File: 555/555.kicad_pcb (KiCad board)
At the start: 2 copper layers, 10 parts, among them J1 Conn_01x03_Pin, U1 LM555xM, U2 TSOP17xx

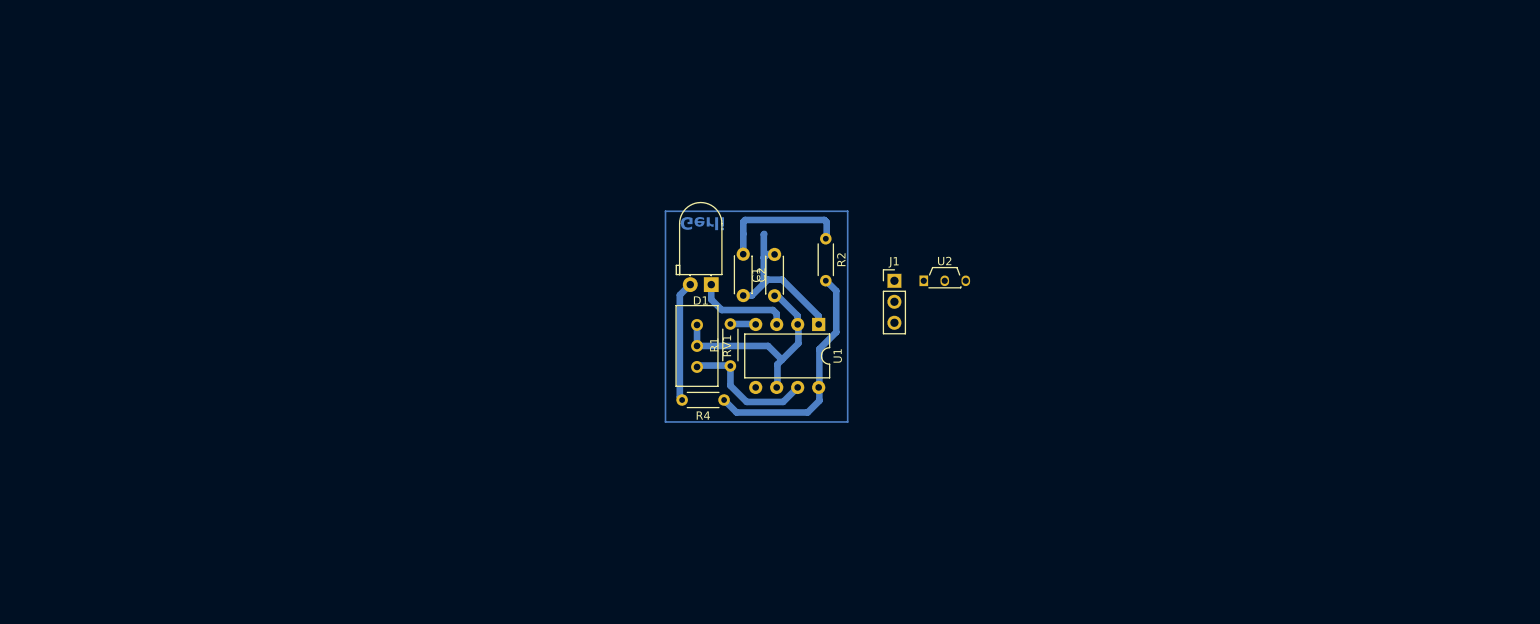
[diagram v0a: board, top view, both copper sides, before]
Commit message: lalalalal
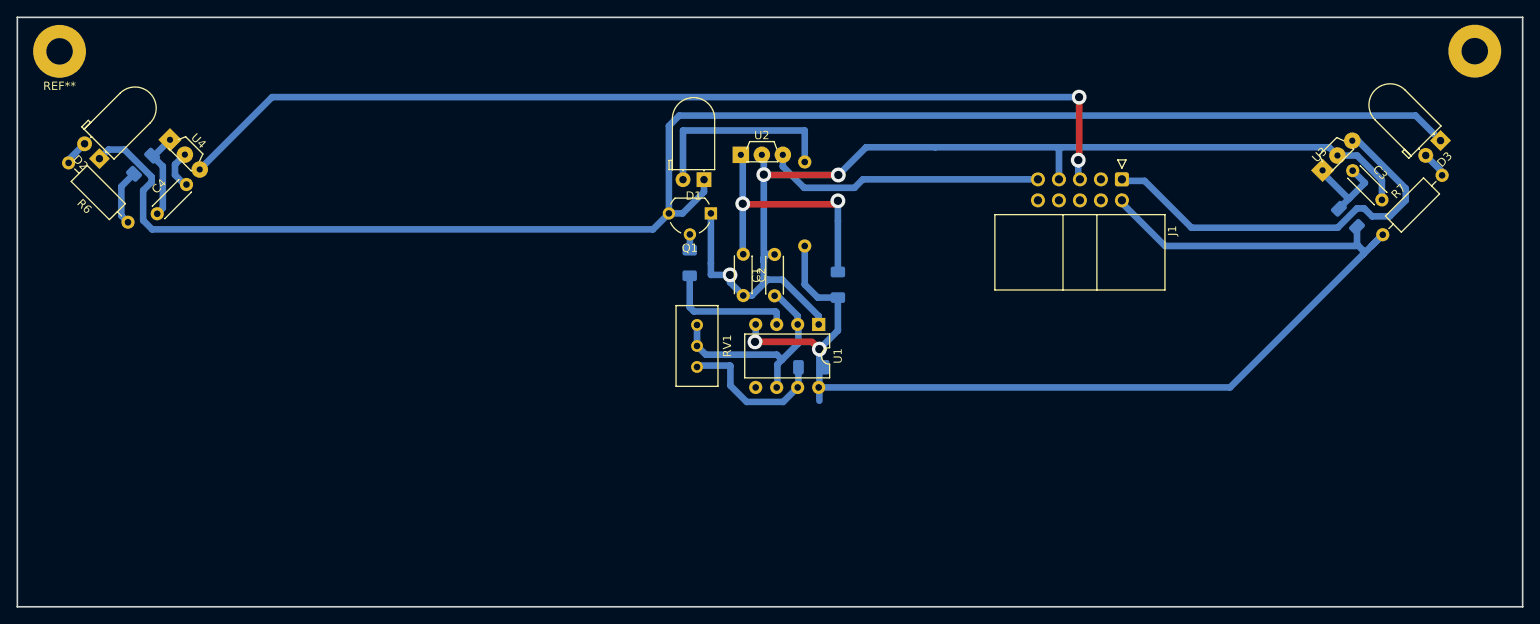
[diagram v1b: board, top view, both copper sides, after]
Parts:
- added ?: , , F.Cu at (210.5, 28.3)
- added C3: 104, Capacitor_THT:C_Disc_D4.3mm_W1.9mm_P5.00mm, F.Cu at (195.7, 42.8)
- added C4: 104, Capacitor_THT:C_Disc_D4.3mm_W1.9mm_P5.00mm, F.Cu at (51.1, 48.0)
- added D2: LED, LED_THT:LED_D5.0mm_Horizontal_O1.27mm_Z3.0mm, F.Cu at (44.1, 41.4)
- added D3: LED, LED_THT:LED_D5.0mm_Horizontal_O1.27mm_Z3.0mm, F.Cu at (206.4, 39.2)
- added Q1: BC547, Package_TO_SOT_THT:TO-92_Wide, F.Cu at (118.1, 48.0)
- added R3: 4.7k, Resistor_SMD:R_1206_3216Metric_Pad1.30x1.75mm_HandSolder, B.Cu at (115.5, 54.0)
- added R5: 100, Resistor_SMD:R_1206_3216Metric_Pad1.30x1.75mm_HandSolder, B.Cu at (195.1, 48.5)
- added R6: 100, Resistor_THT:R_Axial_DIN0207_L6.3mm_D2.5mm_P10.16mm_Horizontal, F.Cu at (47.5, 49.0)
- added R7: 100, Resistor_THT:R_Axial_DIN0207_L6.3mm_D2.5mm_P10.16mm_Horizontal, F.Cu at (199.4, 50.6)
- added R8: 100, Resistor_SMD:R_1206_3216Metric_Pad1.30x1.75mm_HandSolder, B.Cu at (49.3, 42.1)
- added REF**: MountingHole_3.2mm_M3_Pad, MountingHole:MountingHole_3.2mm_M3_Pad, F.Cu at (39.2, 28.4)
- added U3: TSOP17xx, Package_TO_SOT_THT:TO-92S_Wide, F.Cu at (192.1, 42.8)
- added U4: TSOP17xx, Package_TO_SOT_THT:TO-92S_Wide, F.Cu at (52.6, 39.1)
- J1: value Conn_01x03_Pin -> Conn_02x05_Counter_Clockwise; footprint Connector_PinHeader_2.54mm:PinHeader_1x03_P2.54mm_Vertical -> Connector_IDC:IDC-Header_2x05_P2.54mm_Horizontal
- R1, R2: footprint Resistor_THT:R_Axial_DIN0204_L3.6mm_D1.6mm_P5.08mm_Horizontal -> Resistor_SMD:R_1206_3216Metric_Pad1.30x1.75mm_HandSolder; moved to B.Cu
- R4: footprint Resistor_THT:R_Axial_DIN0204_L3.6mm_D1.6mm_P5.08mm_Horizontal -> Resistor_THT:R_Axial_DIN0207_L6.3mm_D2.5mm_P10.16mm_Horizontal; moved to B.Cu
- moved J1 30.1 mm to (167.8, 43.9), turned to -90 degrees
- moved U2 26.9 mm to (121.7, 40.9)
- moved R4 21.0 mm to (129.4, 51.9), turned to 90 degrees
- moved D1 12.7 mm to (117.2, 43.9)
- moved R1 9.78 mm to (130.2, 66.6), turned to 0 degrees
- moved R2 5.76 mm to (133.4, 56.6)
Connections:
- D1 pad 1: Net-(D1-K) -> 38khz
- J1 pad 1: +5V -> Sensores_2
- J1 pad 2: GND -> +5V
- J1 pad 3: Sensores -> unconnected-(J1-Pin_3-Pad3)
- U1 pad 3: Net-(D1-K) -> Net-(U1-Q)
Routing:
- net 38khz: track 0.00 -> 191.3 mm
- net +5V: track 31.7 -> 152.4 mm, vias 0 -> 2
- net Sensores_3: track 0.00 -> 120.1 mm, vias 0 -> 2
- net GND: track 20.4 -> 132.6 mm, vias 0 -> 3
- net Sensores_2: track 0.00 -> 49.2 mm
- net Sensores: track 0.00 -> 33.8 mm
- net Net-(U2-GND): track 16.2 -> 32.6 mm, vias 0 -> 2
- net Net-(U1-Q): track 0.00 -> 16.0 mm
- net Net-(D1-K): track 11.7 -> 0.00 mm
- net Net-(U3-GND): track 0.00 -> 11.3 mm
- net Net-(U4-GND): track 0.00 -> 11.0 mm
- net Net-(D1-A): track 14.5 -> 24.5 mm
- net Net-(D3-A): track 0.00 -> 3.23 mm
- net Net-(D2-A): track 0.00 -> 3.11 mm
- net Net-(U1-DIS): track 16.3 -> 18.8 mm
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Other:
- board outline added: 182.1 x 71.3 mm
- board text removed: "Gerli"
